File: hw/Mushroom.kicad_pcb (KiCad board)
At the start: 2 copper layers, 30 x 30 mm, 28 parts, among them J1 USB_C_Receptacle_PowerOnly_6P, J2 Conn_01x03, J3 Conn_01x12, J4 Conn_01x04, U1 STM32G030F6Px, U2 LPS22HH, U3 SHT30-DIS, U4 BH1750FVI-TR, U5 SPX3819M5-L-3-3

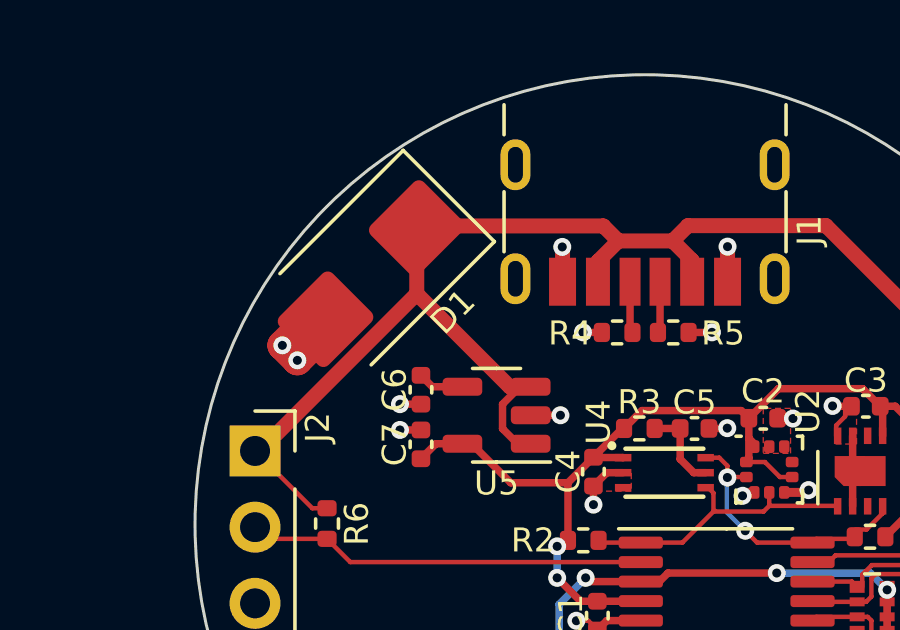
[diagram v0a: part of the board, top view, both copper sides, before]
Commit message: 🎉 Submit for fab (Rev. 1)
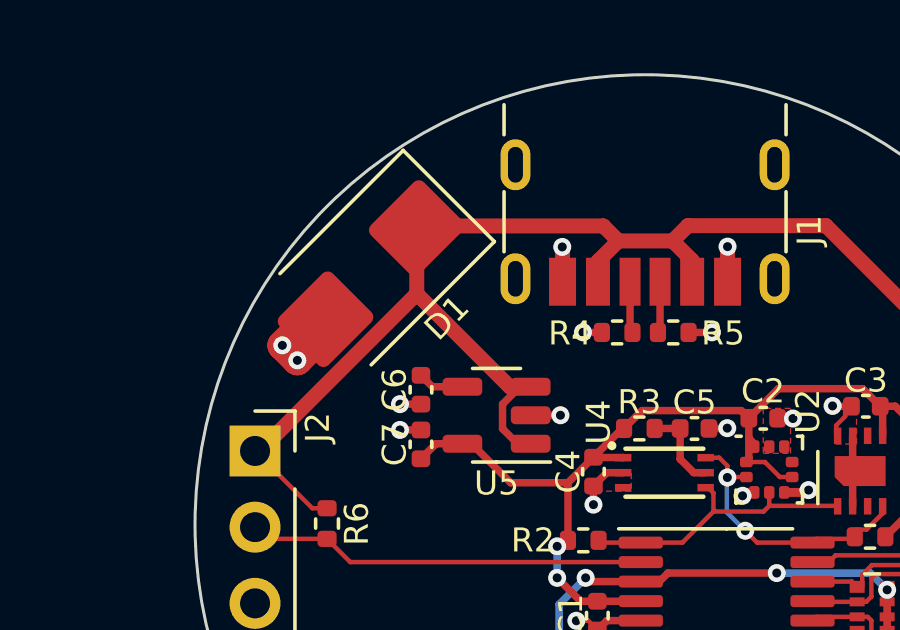
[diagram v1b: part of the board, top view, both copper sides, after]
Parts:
- moved G*** 0.20 mm to (74.1, 51.9)
- moved G*** 0.20 mm to (79.1, 51.7)
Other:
- board text added: "To build resulting board: - Round tracks - Change tolerances to 0.1 mm - Add teardrops - Refill, DRC"
